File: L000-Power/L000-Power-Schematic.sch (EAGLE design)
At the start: 71 parts, among them IC1 LM7805, IC2 LM7905, IC3 LM7809, IC4 LM7909, X1 JST-XH-2PIN, X10 JST-XH-5PIN, X11 JST-XH-5PIN, X12 JST-XH-5PIN, X13 JST-XH-5PIN, X14 JST-XH-5PIN, X15 JST-XH-5PIN, X16 JST-XH-5PIN, X17 JST-XH-5PIN, X18 JST-XH-5PIN, X19 JST-XH-5PIN, X2 JST-XH-5PIN, X20 JST-XH-5PIN, X21 JST-XH-5PIN, X3 JST-XH-5PIN, X4 JST-XH-5PIN, X5 JST-XH-5PIN, X6 JST-XH-5PIN, X7 JST-XH-5PIN, X8 JST-XH-5PIN, X9 JST-XH-5PIN

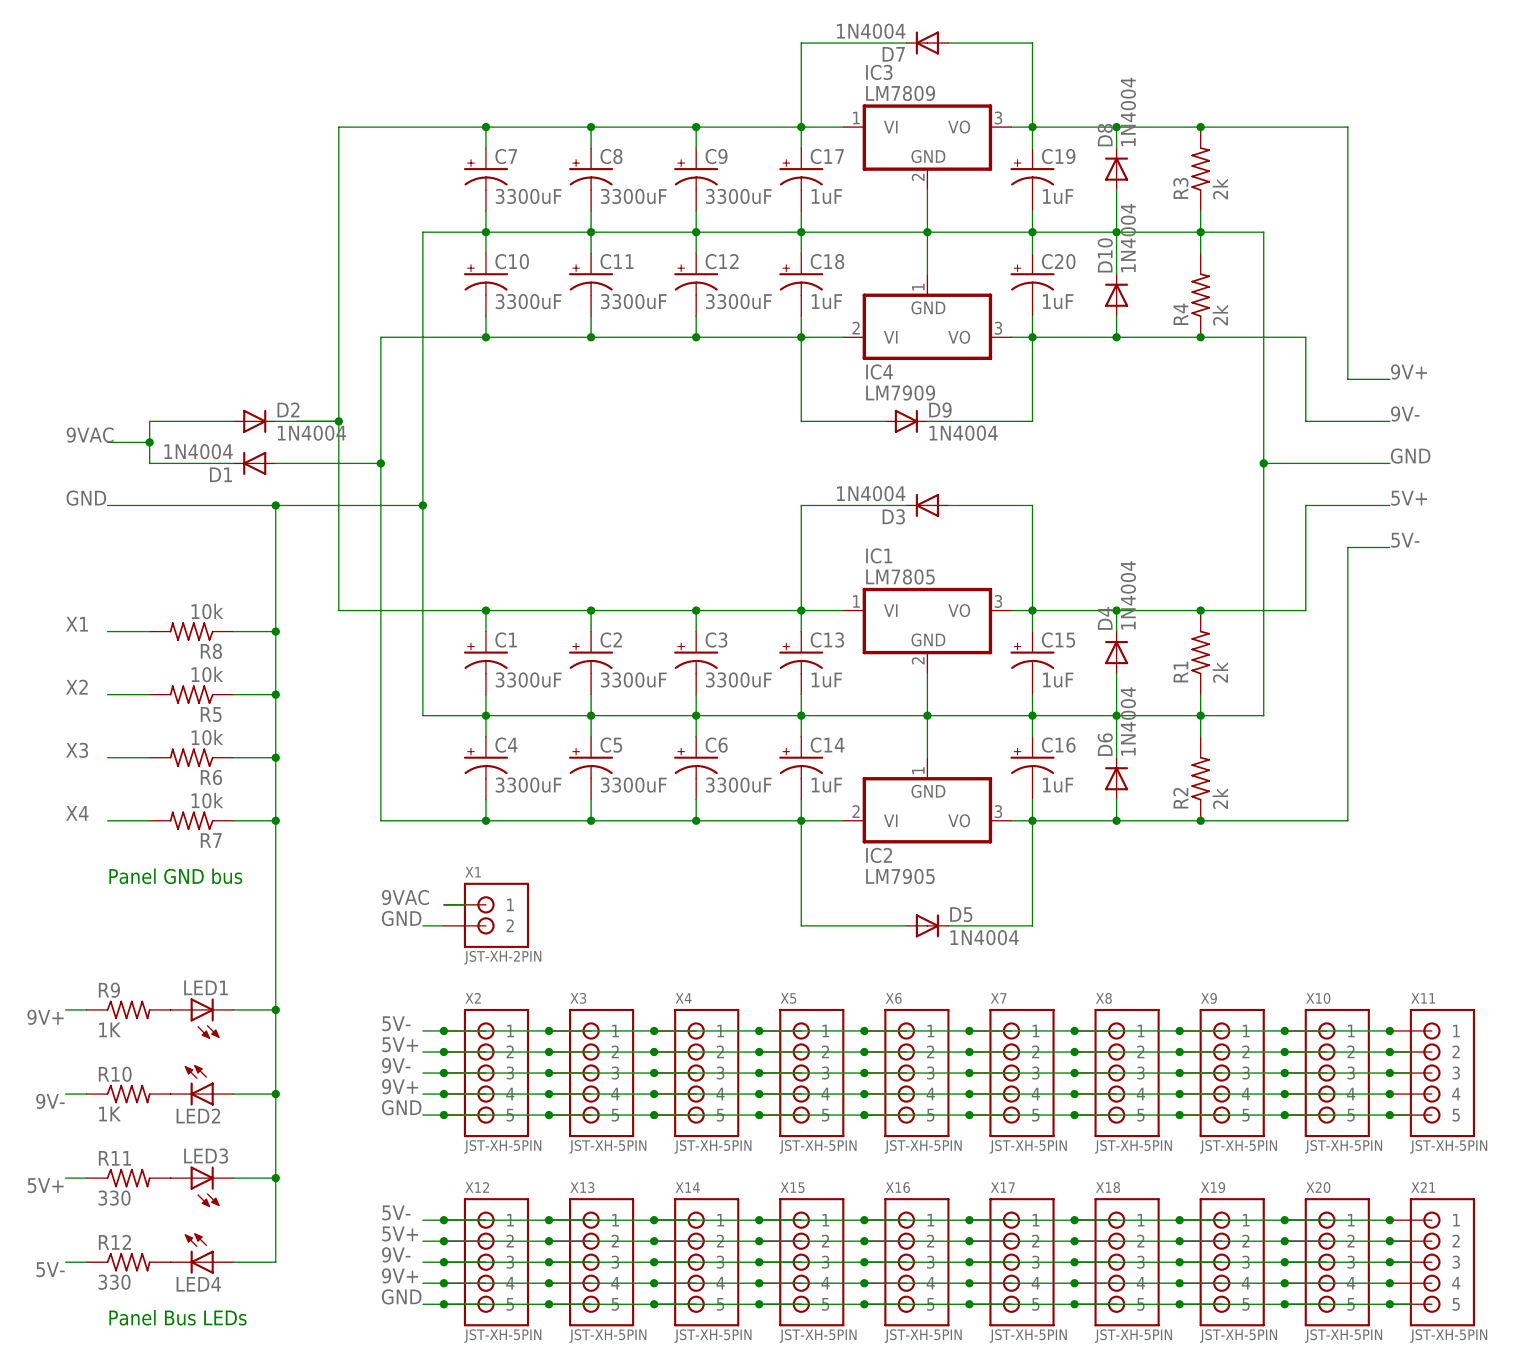
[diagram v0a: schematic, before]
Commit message: FIX V2
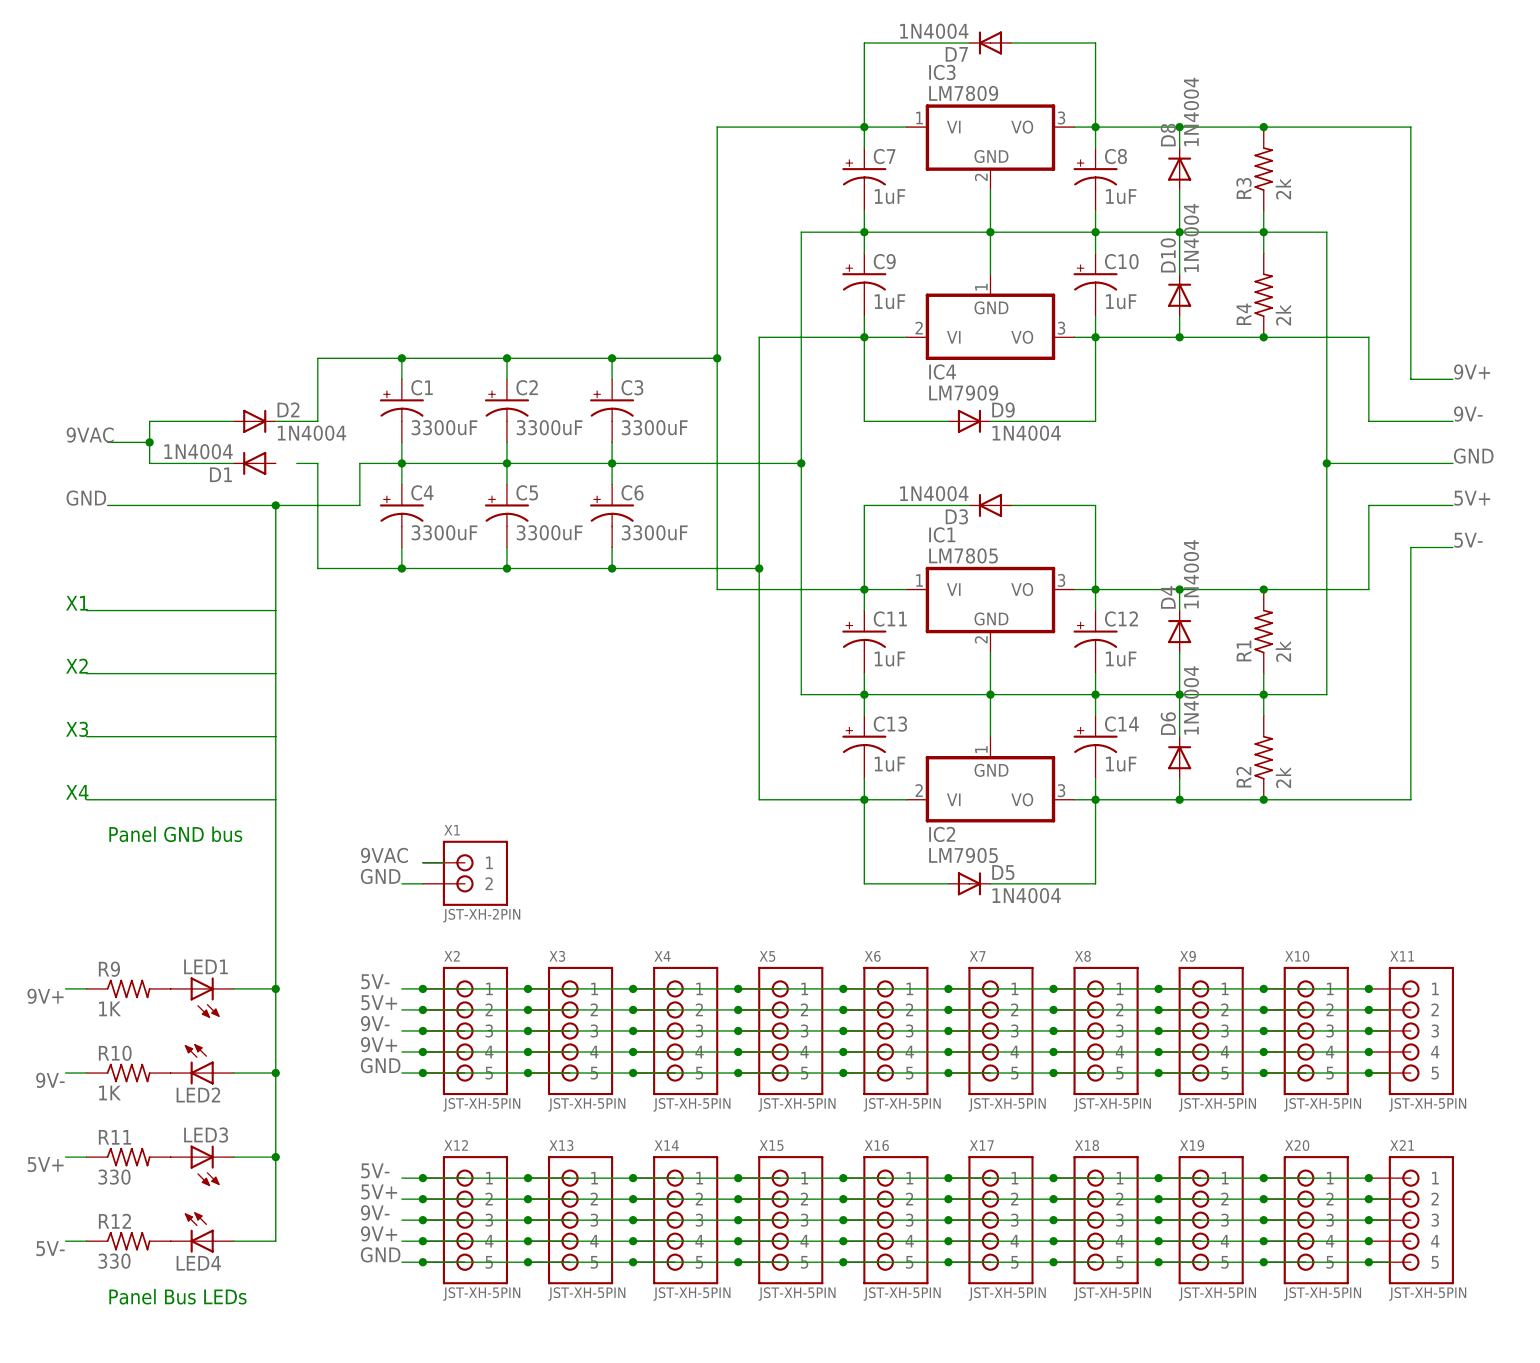
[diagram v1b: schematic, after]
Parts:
- removed C15, C16, C17, C18, C19, C20: 1uF, rcl:CPOL-USE2,5-6E
- removed R5, R6, R7, R8: 10k, resistor:R-US_0309/10
- C10, C11, C12, C7, C8, C9: value 3300uF -> 1uF; device resistor:CPOL-USE5-13 -> rcl:CPOL-USE2,5-6E
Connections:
- removed net N$1: C10.-, C11.-, C12.-, C14.-, C18.-, C4.-, C5.-, C6.-, D1.A, D5.A, D9.A, IC2.VI, IC4.VI
- removed net N$8: C1.+, C13.+, C17.+, C2.+, C3.+, C7.+, C8.+, C9.+, D2.C, D3.C, D7.C, IC1.VI, IC3.VI
- removed net X1: R8.2
- removed net X2: R5.2
- removed net X3: R6.2
- removed net X4: R7.2
- new net N$14: C13.-, C4.-, C5.-, C6.-, C9.-, D5.A, D9.A, IC2.VI, IC4.VI
- new net N$7: C1.+, C11.+, C2.+, C3.+, C7.+, D2.C, D3.C, D7.C, IC1.VI, IC3.VI
- net 5V+: now also C12.+; no longer C15.+
- net 5V-: now also C14.-; no longer C16.-
- net 9V+: now also C8.+; no longer C19.+
- net 9V-: now also C10.-; no longer C20.-
- net GND: now also C11.-, C12.-, C13.+, C9.+; no longer C11.+, C12.+, C13.-, C15.-, C16.+, C17.-, C18.+, C19.-, C20.+, C9.-, R5.1, R6.1, R7.1, R8.1
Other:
- note added: "X1"
- note added: "X2"
- note added: "X3"
- note added: "X4"
- moved on the sheet: C1, C10, C11, C12, C13, C14, C2, C3, C4, C5, C6, C7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
